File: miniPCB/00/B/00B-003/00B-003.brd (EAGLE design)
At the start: 26 parts, among them U1 INA290, U2 AP3012

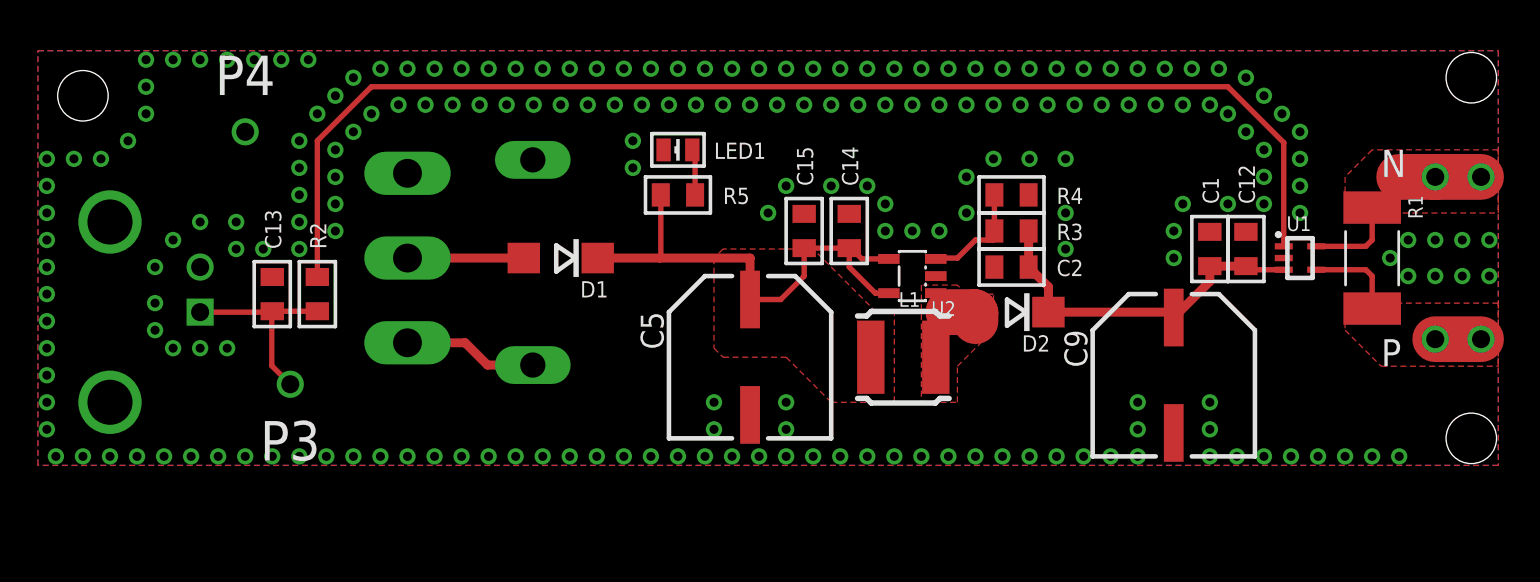
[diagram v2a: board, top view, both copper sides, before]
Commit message: Attempting to fix my Git merge error.
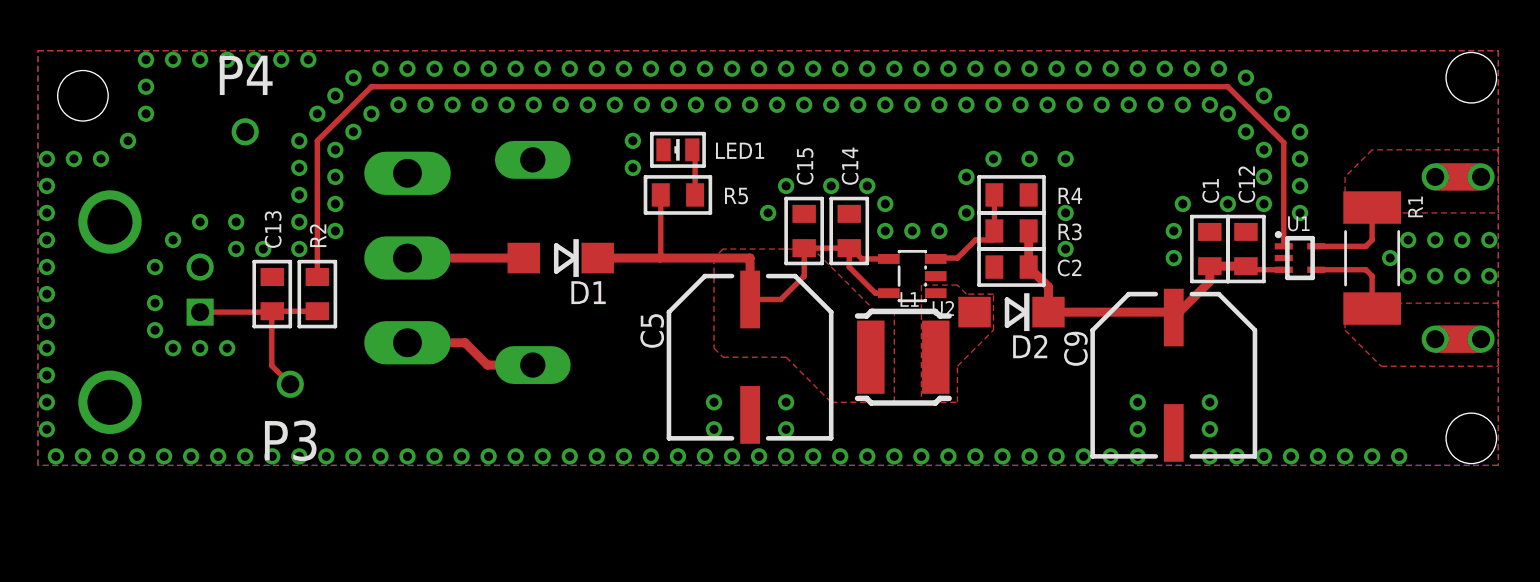
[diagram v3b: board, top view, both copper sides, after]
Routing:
- net N: track 9.58 -> 5.04 mm
- net P: track 7.58 -> 5.04 mm
- net HV_SW: track 1.97 -> 0.00 mm
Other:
- board text removed: "B1"
- board text removed: "C1"
- board text removed: "C12"
- board text removed: "C13"
- board text removed: "C14"
- board text removed: "C15"
- board text removed: "C2"
- board text removed: "C5"
- board text removed: "C9"
- board text removed: "D1"
- board text removed: "D2"
- board text removed: "J1"
- board text removed: "L1"
- board text removed: "LED1"
- board text removed: "N"
- board text removed: "P"
- board text removed: "P3"
- board text removed: "P4"
- board text removed: "R1"
- board text removed: "R2"
- board text removed: "R3"
- board text removed: "R4"
- board text removed: "R5"
- board text removed: "U1"
- board text removed: "U2"
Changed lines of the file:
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@@
 <layer number="123" name="tTestmark" color="7" fill="1" visible="yes" active="yes"/>
 <layer number="124" name="bTestmark" color="7" fill="1" visible="yes" active="yes"/>
-<layer number="125" name="_tNames" color="14" fill="1" visible="yes" active="yes"/>
-<layer number="126" name="_bNames" color="5" fill="1" visible="yes" active="yes"/>
+<layer number="125" name="_tNames" color="7" fill="1" visible="yes" active="yes"/>
+<layer number="126" name="_bNames" color="7" fill="1" visible="yes" active="yes"/>
 <layer number="127" name="_tValues" color="7" fill="1" visible="yes" active="yes"/>
 <layer number="128" name="_bValues" color="7" fill="1" visible="yes" active="yes"/>
@@
 <wire x1="48.5" y1="4.5" x2="52.5" y2="4.5" width="0.5" layer="41"/>
 <wire x1="52.5" y1="4.5" x2="56" y2="8" width="0.5" layer="41"/>
-<wire x1="56" y1="8" x2="56" y2="11" width="0.5" layer="41"/>
-<wire x1="56" y1="11" x2="47.5" y2="11" width="0.5" layer="41"/>
+<wire x1="56" y1="8" x2="56" y2="10.5" width="0.5" layer="41"/>
+<wire x1="56" y1="10.5" x2="52.5" y2="10.5" width="0.5" layer="41"/>
+<wire x1="52.5" y1="10.5" x2="52" y2="11" width="0.5" layer="41"/>
+<wire x1="52" y1="11" x2="47.5" y2="11" width="0.5" layer="41"/>
 <wire x1="82" y1="19" x2="75" y2="19" width="0.3" layer="41"/>
 <wire x1="75" y1="19" x2="73" y2="17" width="0.3" layer="41"/>
@@
 <wire x1="73" y1="10.5" x2="82" y2="10.5" width="0.3" layer="42"/>
 <wire x1="55" y1="15" x2="55" y2="11" width="0.3" layer="41"/>
-<text x="75.5" y="6.5" size="1.5" layer="21" font="vector" ratio="12">P</text>
-<text x="75.5" y="17" size="1.5" layer="21" font="vector" ratio="12">N</text>
-<text x="26.499996875" y="24.000003125" size="1.27" layer="126" font="vector" rot="MR180">B1</text>
-<text x="66.49999375" y="15.49999375" size="0.899996875" layer="125" font="vector" ratio="13" rot="R90">C1</text>
-<text x="57.5000125" y="11.500003125" size="0.899996875" layer="125" font="vector" ratio="13">C2</text>
-<text x="35.706" y="9.524009375" size="1.27" layer="125" font="vector" ratio="12" rot="R270" align="top-left">C5</text>
-<text x="59.206003125" y="8.5240125" size="1.27" layer="125" font="vector" ratio="12" rot="R270" align="top-left">C9</text>
-<text x="68.499990625" y="15.49999375" size="0.899996875" layer="125" font="vector" ratio="13" rot="R90">C12</text>
-<text x="14.499996875" y="13" size="0.899996875" layer="125" font="vector" ratio="13" rot="R90">C13</text>
-<text x="46.500009375" y="16.49999375" size="0.899996875" layer="125" font="vector" ratio="13" rot="R90">C14</text>
-<text x="43.9999875" y="16.49999375" size="0.899996875" layer="125" font="vector" ratio="13" rot="R90">C15</text>
-<text x="32.639990625" y="11.213996875" size="0.899996875" layer="125" font="vector" ratio="10" rot="R180">D1</text>
-<text x="57.13999375" y="8.214003125" size="0.899996875" layer="125" font="vector" ratio="10" rot="R180">D2</text>
-<text x="12" y="2.49999375" size="1.499996875" layer="126" font="vector" ratio="12" rot="MR90">J1</text>
-<text x="48.746003125" y="9.7940125" size="0.8128" layer="125" font="vector">L1</text>
-<text x="38.5" y="17.999990625" size="0.899996875" layer="125" font="vector" ratio="12">LED1</text>
-<text x="14.999996875" y="3.4599875" size="2.1844" layer="125" font="vector" ratio="12" rot="R180" align="bottom-center">P3</text>
-<text x="12.5" y="21.5399875" size="2.1844" layer="125" font="vector" ratio="12" align="bottom-center">P4</text>
-<text x="76.999996875" y="15.99999375" size="0.8128" layer="125" font="vector" ratio="12" rot="R270">R1</text>
-<text x="16.999990625" y="13" size="0.899996875" layer="125" font="vector" ratio="13" rot="R90">R2</text>
-<text x="57.5000125" y="13.499996875" size="0.899996875" layer="125" font="vector" ratio="13">R3</text>
-<text x="57.5000125" y="15.49999375" size="0.899996875" layer="125" font="vector" ratio="13">R4</text>
-<text x="38.999996875" y="15.49999375" size="0.899996875" layer="125" font="vector" ratio="13">R5</text>
-<text x="70.25" y="13.999996875" size="0.8128" layer="125" font="vector" ratio="12">U1</text>
-<text x="51.913003125" y="10.103003125" size="0.8128" layer="125" font="vector" rot="R180">U2</text>
 </plain>
 <attributes>
@@
 <element name="U1" library="nolan-utsa" package="SC70-5" value="INA290" x="71" y="12.5" smashed="yes" rot="R270">
 <attribute name="NAME" x="70.25" y="14" size="0.8128" layer="25" font="vector" ratio="12"/>
+<attribute name="VALUE" x="71" y="10.5" size="0.8128" layer="27" font="vector" ratio="12" align="center"/>
 </element>
 <element name="P1" library="nolan-utsa" package="PINS_1_1MM" value="" x="78.5" y="8" smashed="yes"/>
@@
 </element>
 <element name="D2" library="minipcb" package="DO214AC" value="1N5819" x="55" y="9.5" smashed="yes" rot="R180">
-<attribute name="NAME" x="57.14" y="8.214" size="0.9" layer="25" font="vector" ratio="10" rot="R180"/>
+<attribute name="NAME" x="57.14" y="8.214" size="1.27" layer="25" font="vector" ratio="10" rot="R180"/>
+<attribute name="VALUE" x="57.64" y="12.056" size="1.27" layer="27" ratio="10" rot="R180"/>
 </element>
 <element name="D1" library="minipcb" package="DO214AC" value="1N5819" x="30" y="12.5" smashed="yes" rot="R180">
-<attribute name="NAME" x="32.64" y="11.214" size="0.9" layer="25" font="vector" ratio="10" rot="R180"/>
+<attribute name="NAME" x="32.64" y="11.214" size="1.27" layer="25" ratio="10" rot="R180"/>
+<attribute name="VALUE" x="32.64" y="15.056" size="1.27" layer="27" ratio="10" rot="R180"/>
 </element>
 <element name="J1" library="minipcb" package="BNC_RIGHTANGLE" value="" x="10" y="9.5" smashed="yes" rot="MR270">
@@
 <element name="R1" library="minipcb" package="R2512K" value="0R5" x="75" y="12.5" smashed="yes" rot="R270">
 <attribute name="NAME" x="77" y="16" size="0.8128" layer="25" font="vector" ratio="12" rot="R270"/>
+<attribute name="VALUE" x="73" y="9" size="0.8128" layer="27" font="vector" ratio="12" rot="R90"/>
 </element>
 <element name="C1" library="minipcb" package="C0805" value="1u" x="66" y="13" smashed="yes" rot="R90">
@@
 <contactref element="R1" pad="2"/>
 <wire x1="75" y1="9.7" x2="75" y2="11.5" width="0.3" layer="1"/>
-<wire x1="81.04" y1="8" x2="78.5" y2="8" width="2.54" layer="1"/>
 </signal>
 <signal name="N">
@@
 <contactref element="R1" pad="1"/>
 <wire x1="75" y1="13.5" x2="75" y2="15.3" width="0.3" layer="1"/>
-<wire x1="78.5" y1="17" x2="76.5" y2="17" width="2.54" layer="1"/>
-<wire x1="81.04" y1="17" x2="78.5" y2="17" width="2.54" layer="1"/>
+<wire x1="78.5" y1="17" x2="81.04" y2="17" width="0" layer="19" extent="1-1"/>
 </signal>
 <signal name="GND">
@@
 <vertex x="52" y="11"/>
 </polygon>
-<wire x1="52.95" y1="9.5" x2="51.5" y2="9.5" width="2.54" layer="1"/>
-<wire x1="52.95" y1="9.5" x2="53" y2="9.45" width="2.54" layer="1"/>
-<wire x1="53" y1="9.45" x2="53" y2="9" width="2.54" layer="1"/>
 </signal>
 <signal name="HV_FB">
